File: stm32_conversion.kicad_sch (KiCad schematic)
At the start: 44 parts, among them IC2 LM3940IMP-3.3_NOPB, J2 Micro_SD_Card, U2 TXB0108PW, U3 TXB0108PW, U4 W25Q16JVSS, Y1 Crystal_GND23

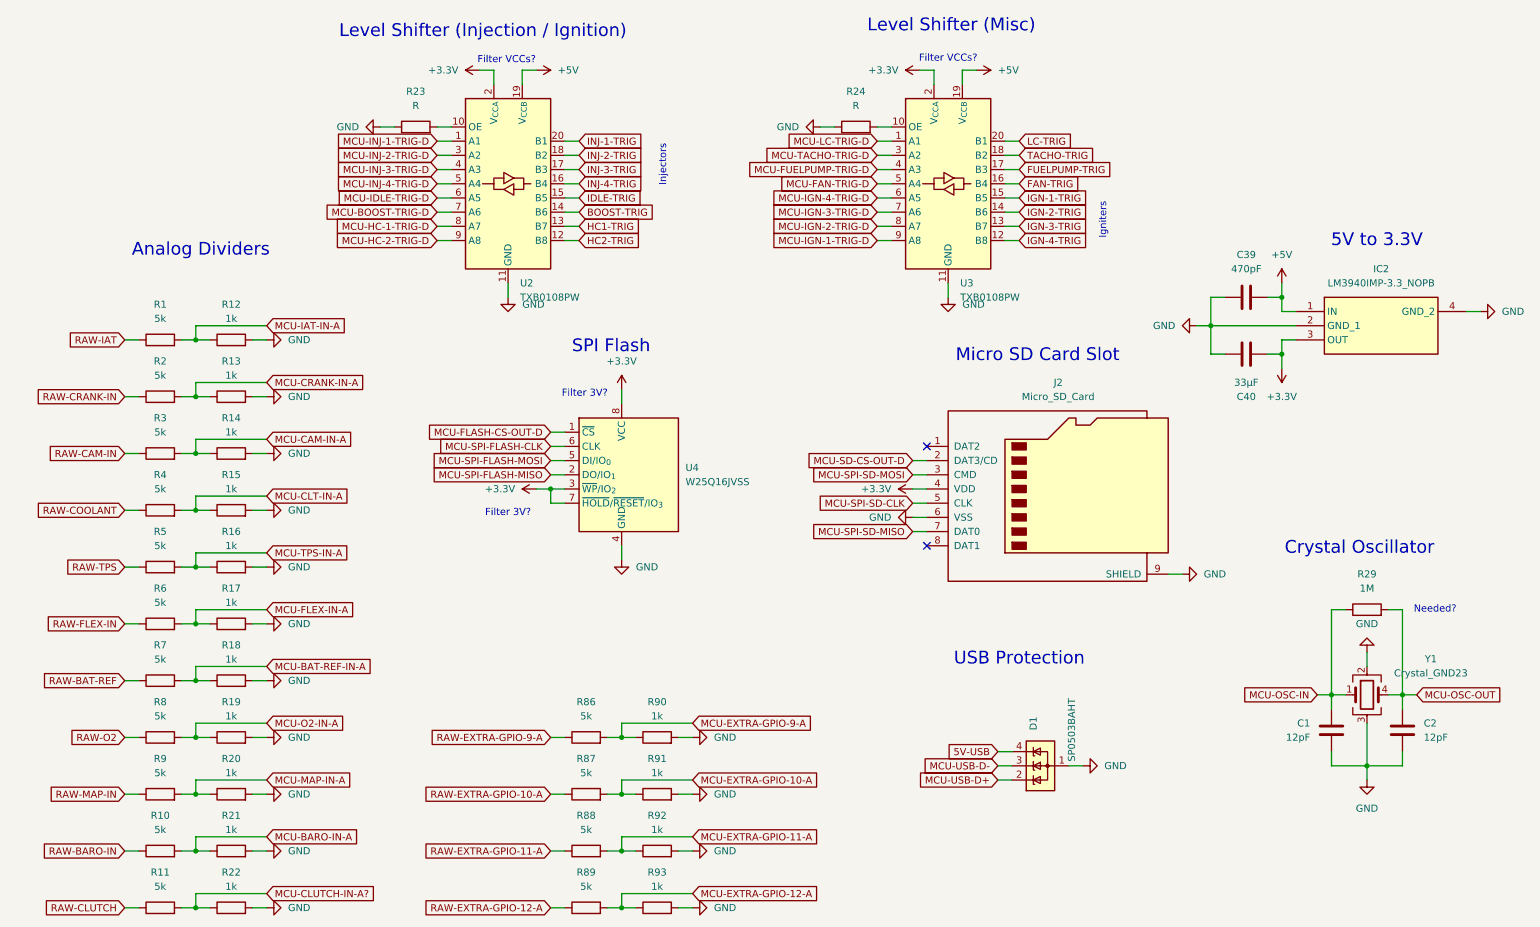
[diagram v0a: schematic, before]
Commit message: Pre MCU switch
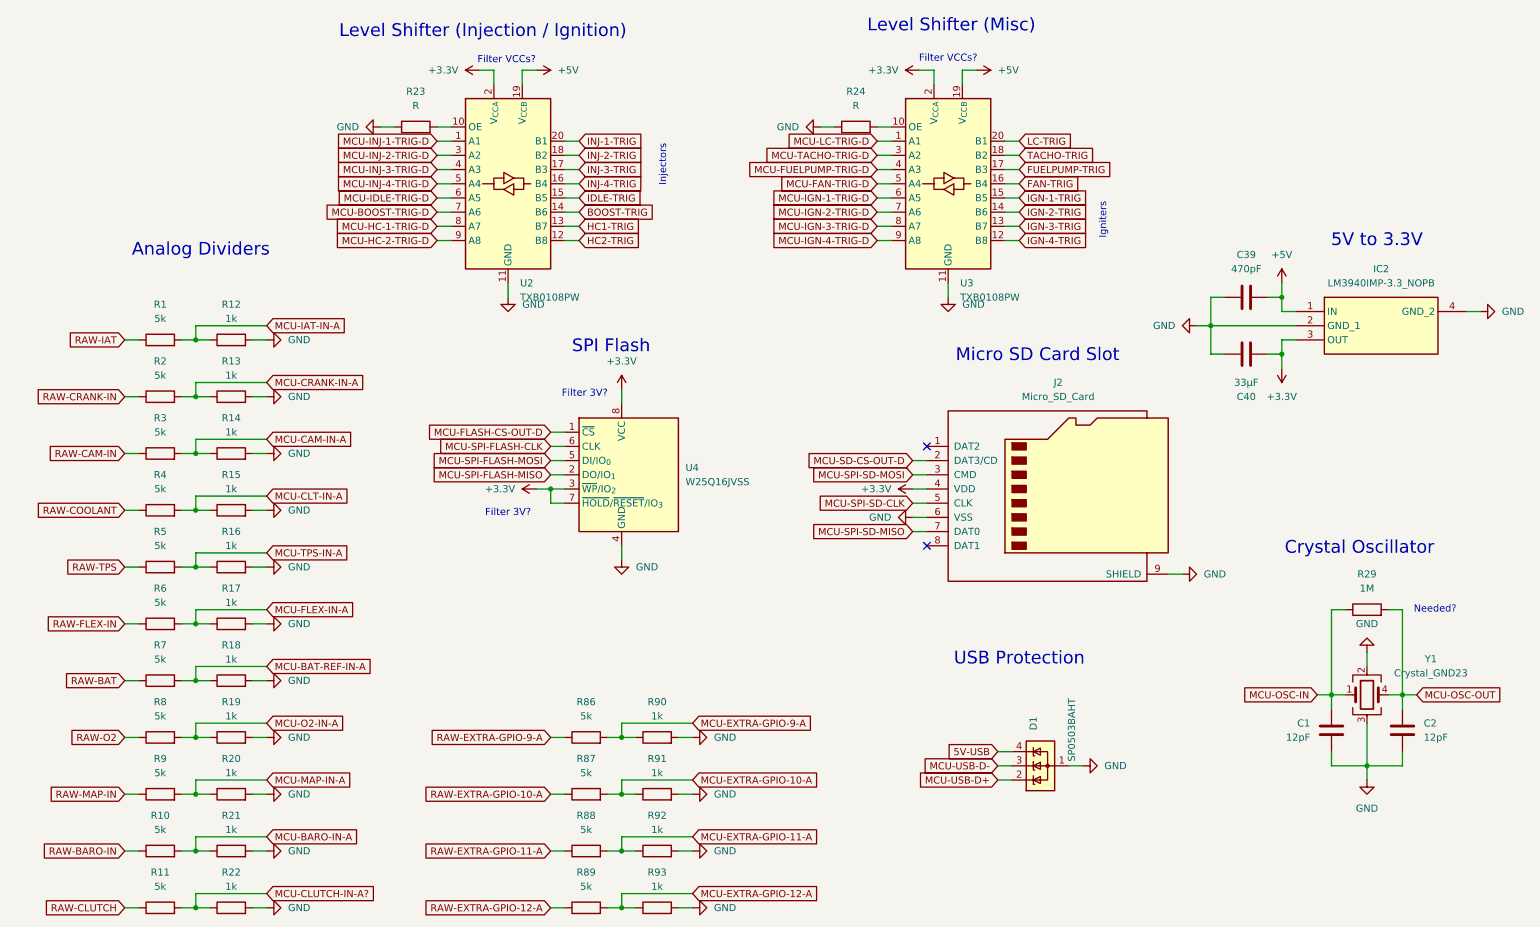
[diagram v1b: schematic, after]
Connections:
- net MCU-IGN-1-TRIG-D: now also U3.6 (A5); no longer U3.9 (A8)
- net MCU-IGN-2-TRIG-D: now also U3.7 (A6); no longer U3.8 (A7)
- net MCU-IGN-3-TRIG-D: now also U3.8 (A7); no longer U3.7 (A6)
- net MCU-IGN-4-TRIG-D: now also U3.9 (A8); no longer U3.6 (A5)
- net RAW-BAT-REF renamed RAW-BAT
